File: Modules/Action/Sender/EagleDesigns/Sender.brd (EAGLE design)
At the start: 100 x 80 mm, 10 parts, among them U2 ATMEGA328P_TQFP

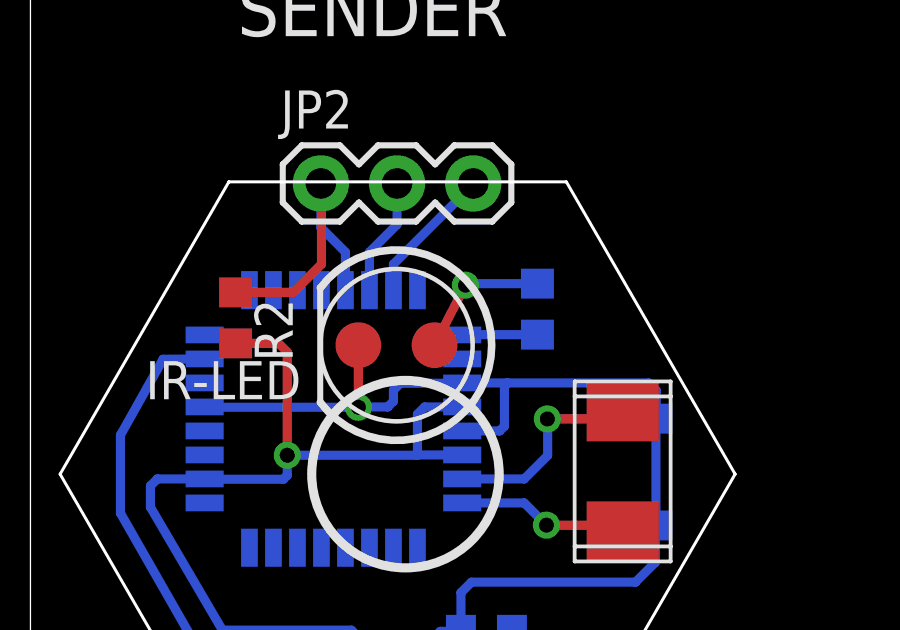
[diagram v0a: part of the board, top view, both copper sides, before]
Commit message: minor organizations
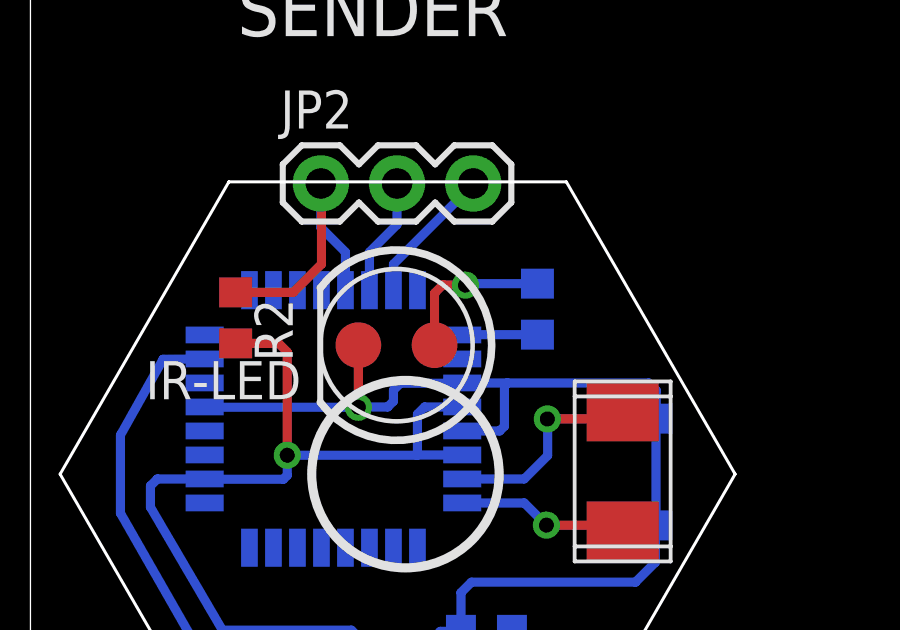
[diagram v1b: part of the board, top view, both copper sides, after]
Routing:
- net N$2: track 4.67 -> 5.30 mm
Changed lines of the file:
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@@
 <wire x1="14.55" y1="17.05" x2="14.5" y2="17" width="0.3048" layer="16"/>
 <via x="14.5" y="17" extent="1-16" drill="0.5"/>
-<wire x1="14.5" y1="17" x2="13.47" y2="15" width="0.3048" layer="1"/>
+<wire x1="13.47" y1="15" x2="13.47" y2="16.73" width="0.3048" layer="1"/>
+<wire x1="13.47" y1="16.73" x2="13.75" y2="17.01" width="0.3048" layer="1"/>
+<wire x1="13.75" y1="17.01" x2="14.49" y2="17.01" width="0.3048" layer="1"/>
+<wire x1="14.49" y1="17.01" x2="14.5" y2="17" width="0.3048" layer="1"/>
 </signal>
 <signal name="IR-OUT">
